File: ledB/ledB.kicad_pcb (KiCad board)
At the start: 2 copper layers, 26 x 34 mm, 6 parts

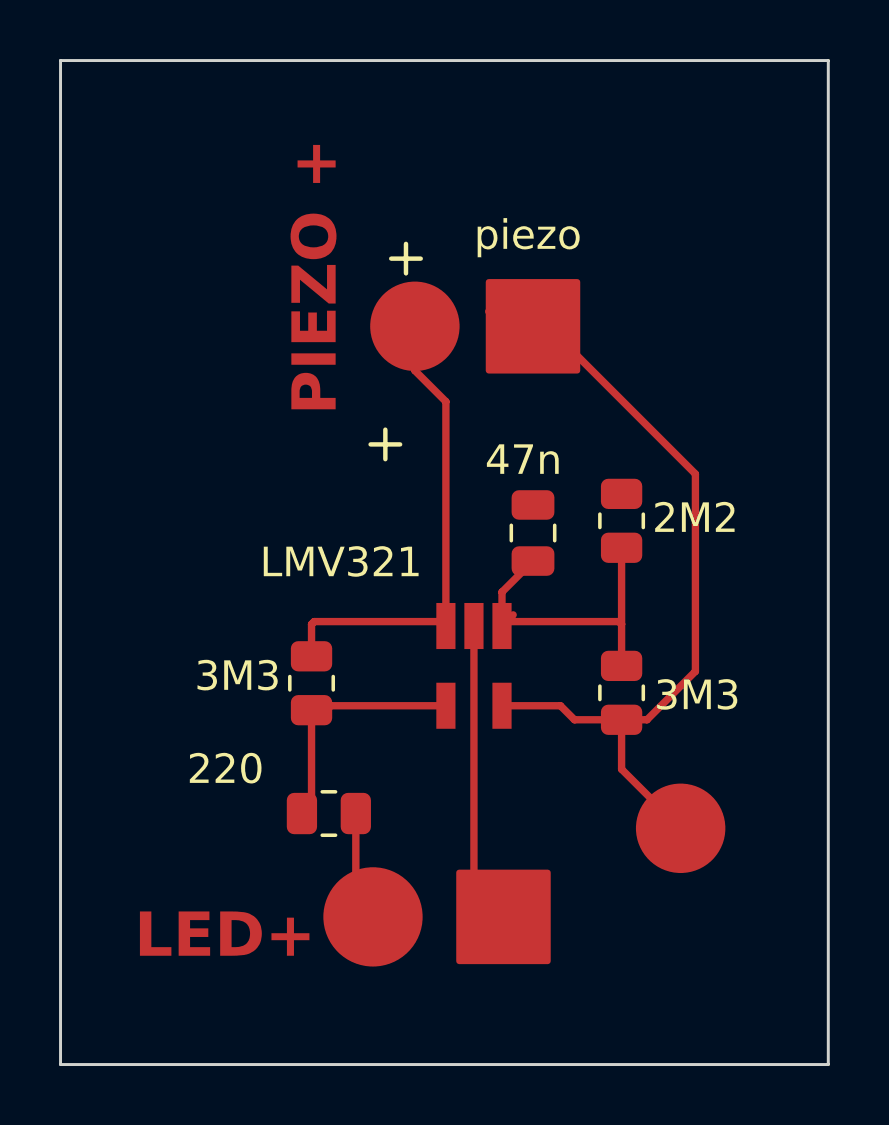
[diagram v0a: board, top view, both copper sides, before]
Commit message: etch
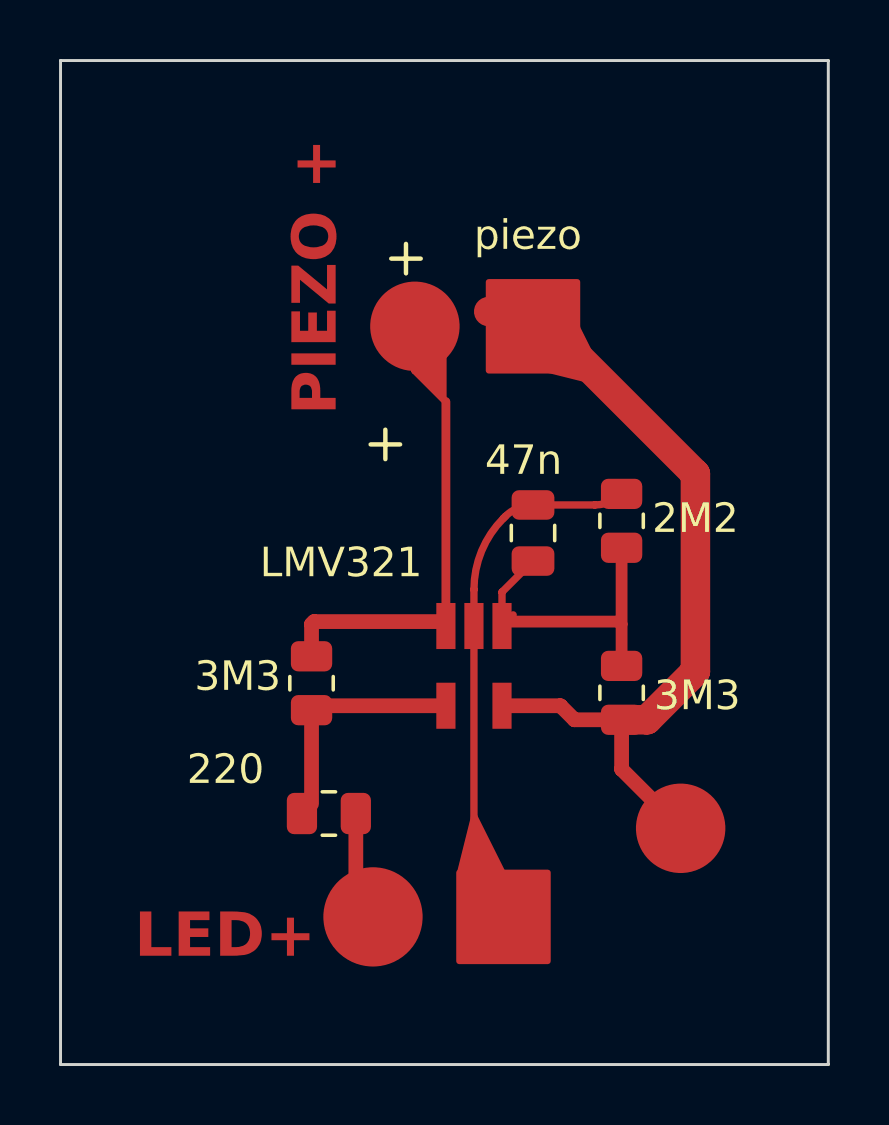
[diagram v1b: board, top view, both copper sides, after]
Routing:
- net GND: track 10.3 -> 18.4 mm
